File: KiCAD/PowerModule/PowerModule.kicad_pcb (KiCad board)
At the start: 2 copper layers, 90 x 70 mm, 39 parts, among them J1 GPU, J2 BATTERY, J3 BUS, J4 MONITOR, J5 MASTER, Q3 AO3401A, Q5 AO3401A, U2 INA219BxDCN, U3 INA219BxDCN, U4 INA219BxDCN, U8 INA219BxDCN

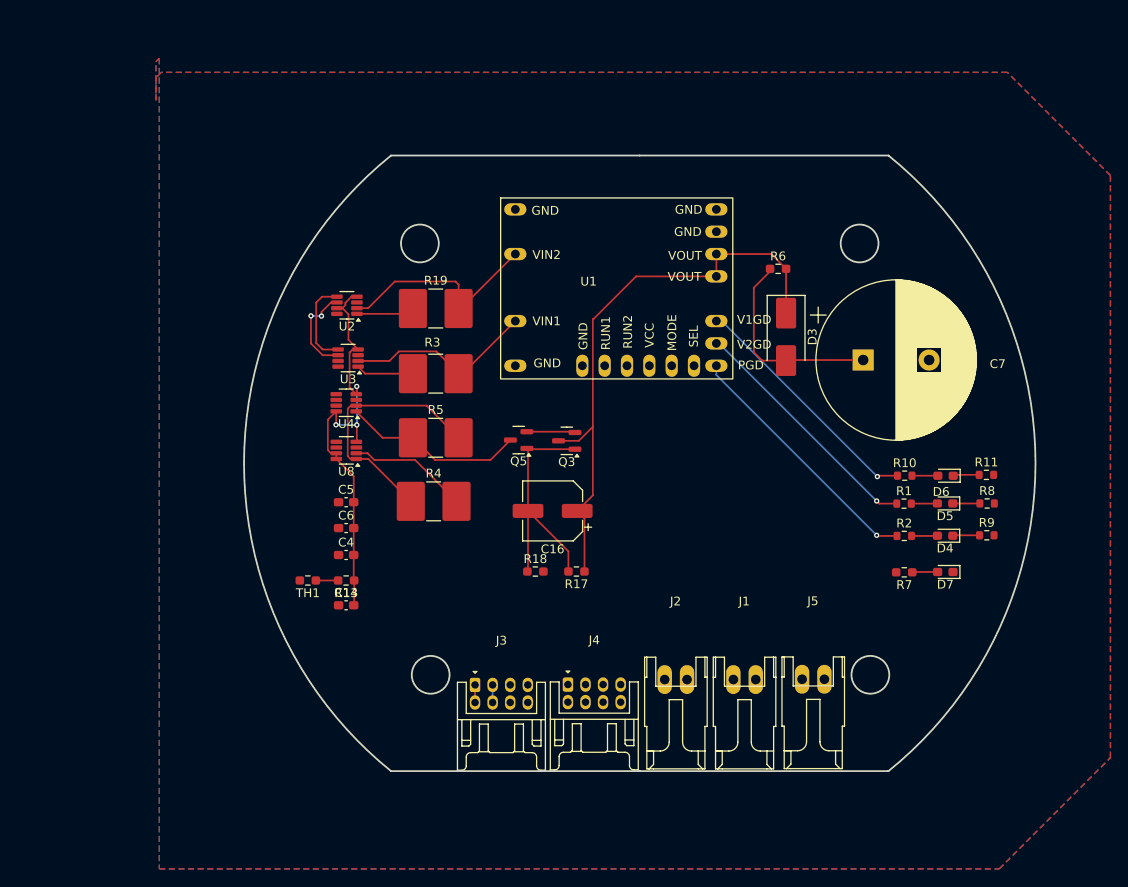
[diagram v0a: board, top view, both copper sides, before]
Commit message: 配線の確認お願いします
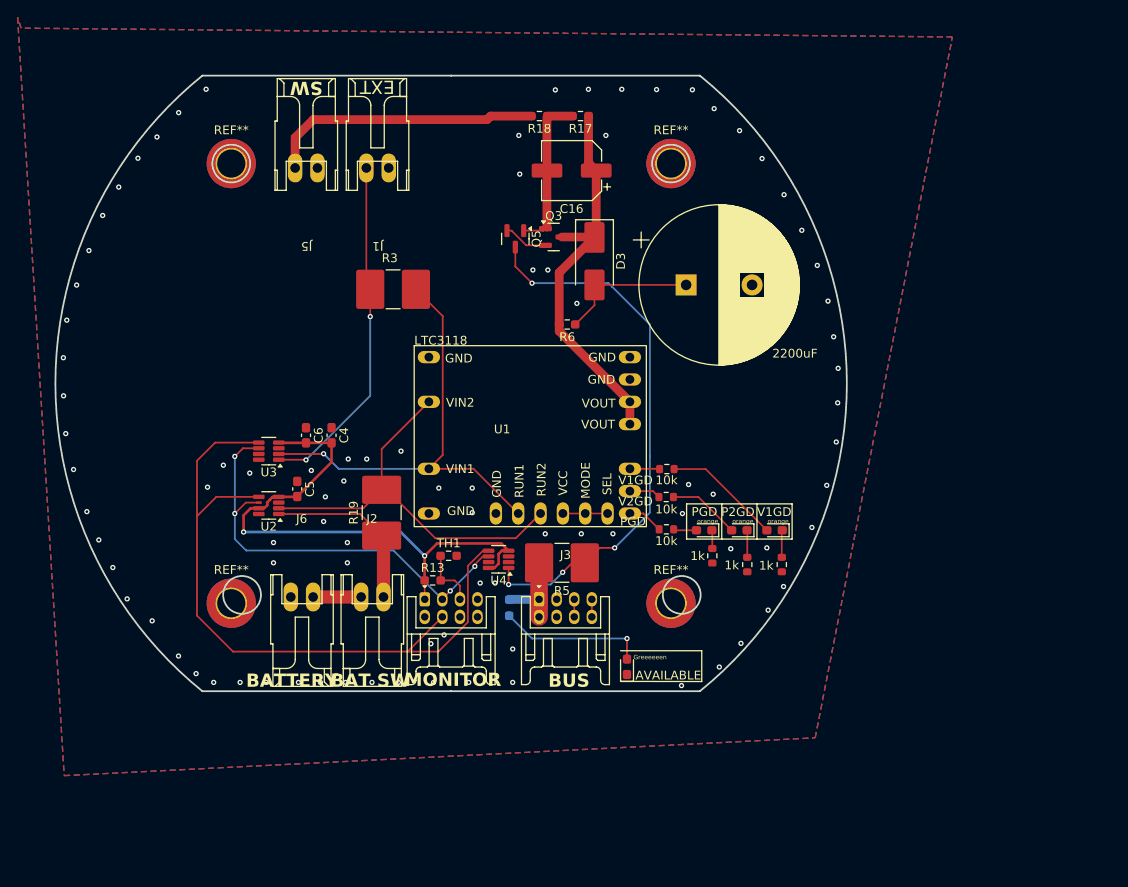
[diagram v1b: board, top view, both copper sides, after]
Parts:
- removed C14: 0.1uF, Capacitor_SMD:C_0603_1608Metric_Pad1.08x0.95mm_HandSolder
- removed R4: 0.1R, Resistor_SMD:R_2816_7142Metric_Pad3.20x4.45mm_HandSolder
- removed U8: INA219BxDCN, Package_TO_SOT_SMD:SOT-23-8
- added J6: Conn_01x02, TSRP_Connector_Hirose:DF1B-2S-2.5R, F.Cu at (133.0, 125.0)
- added REF**: MountingHole_3.2mm_M3_DIN965_Pad_TopBottom, MountingHole:MountingHole_3.2mm_M3_DIN965_Pad_TopBottom, F.Cu at (125.0, 125.0)
- added REF**: MountingHole_3.2mm_M3_DIN965_Pad_TopBottom, MountingHole:MountingHole_3.2mm_M3_DIN965_Pad_TopBottom, F.Cu at (125.0, 75.0)
- added REF**: MountingHole_3.2mm_M3_DIN965_Pad_TopBottom, MountingHole:MountingHole_3.2mm_M3_DIN965_Pad_TopBottom, F.Cu at (175.0, 125.0)
- added REF**: MountingHole_3.2mm_M3_DIN965_Pad_TopBottom, MountingHole:MountingHole_3.2mm_M3_DIN965_Pad_TopBottom, F.Cu at (175.0, 75.0)
- R7: moved to B.Cu
- moved J5 82.8 mm to (133.6, 74.8), turned to 180 degrees
- moved J1 72.7 mm to (141.7, 74.8), turned to 180 degrees
- moved R17 51.8 mm to (164.7, 69.6)
- moved R18 51.8 mm to (160.0, 69.6), turned to 180 degrees
- moved R7 45.1 mm to (156.6, 125.5), turned to 90 degrees
- moved C16 38.8 mm to (163.7, 75.8)
- moved D7 37.8 mm to (170.0, 132.2), turned to 90 degrees
- moved J2 35.8 mm to (141.0, 125.0)
- moved R9 31.3 mm to (179.7, 119.6), turned to -90 degrees
- moved R8 28.1 mm to (183.7, 120.6), turned to -90 degrees
- moved D4 27.4 mm to (178.8, 116.7)
- moved R1 27.1 mm to (174.5, 112.9)
- moved R2 27.1 mm to (174.5, 116.6)
- moved R10 27.1 mm to (174.5, 109.7)
- moved R11 25.4 mm to (187.6, 120.6), turned to -90 degrees
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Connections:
- J2 pad 1: +15V -> Net-(J2-Pin_1)
- R5 pad 2: +VSW -> +12V
- U4 pad 2: +VSW -> +12V
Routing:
- net I2C_SCL: track 10.0 -> 83.3 mm
- net Net-(Q5-S): track 20.8 -> 65.0 mm, vias 0 -> 4
- net I2C_SDA: track 10.6 -> 49.6 mm, vias 2 -> 4
- net Net-(J1-Pin_2): track 6.56 -> 39.6 mm, vias 0 -> 2
- net Net-(J5-Pin_2): track 0.00 -> 31.3 mm
- net Net-(U1-RUN1): track 21.9 -> 52.1 mm, vias 0 -> 1
- net +VSW: track 29.0 -> 0.00 mm
- net Net-(U1-PGD): track 29.2 -> 4.07 mm, vias 1 -> 0
- net Net-(U1-V1GD): track 28.0 -> 3.39 mm, vias 1 -> 0
- net Net-(U1-V2GD): track 28.1 -> 3.58 mm, vias 1 -> 0
- net Net-(D3-K): track 66.8 -> 44.2 mm
- net Net-(U1-RUN2): track 24.7 -> 46.3 mm
- net Net-(D7-A): track 2.90 -> 16.8 mm, vias 0 -> 1
- net +3.3V: track 49.8 -> 63.1 mm, vias 3 -> 2
- net Net-(J2-Pin_2): track 6.62 -> 19.8 mm
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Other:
- board text added: "10k"
- board text added: "1k"
- board text added: "AVAILABLE"
- board text added: "BAT SW"
- board text added: "BATTERY"
- board text added: "BUS"
- board text added: "EXT"
- board text added: "Greeeeeen"
- board text added: "LTC3118"
- board text added: "MONITOR"
- board text added: "P2GD"
- board text added: "PGD"
- board text added: "SW"
- board text added: "V1GD"
- board text added: "orange"
